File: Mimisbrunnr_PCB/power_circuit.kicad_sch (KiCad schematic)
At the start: 4 parts, among them J2 Jack-DC, U2 TLV76733DRVx

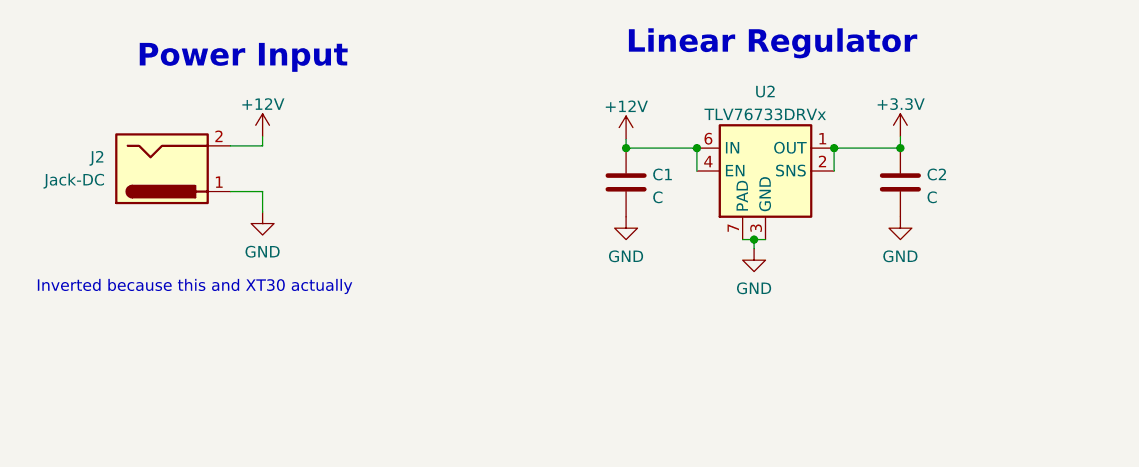
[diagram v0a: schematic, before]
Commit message: routing finished
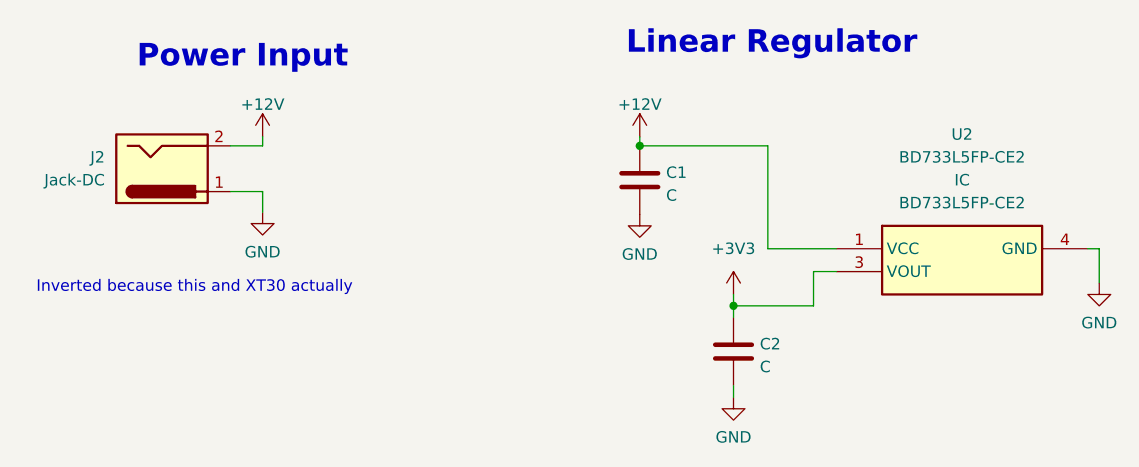
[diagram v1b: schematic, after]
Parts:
- removed U2: TLV76733DRVx, Package_TO_SOT_SMD:SOT-23-5_HandSoldering, symbol Regulator_Linear:TLV76733DRVx
- added U2: BD733L5FP-CE2, BD733L5FP:BD750L5FPCE2, symbol BD733L5FP:BD733L5FP-CE2
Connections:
- net +12V: now also U2.1 (VCC)
- net +3V3: now also U2.3 (VOUT)
- net GND: now also U2.4 (GND)
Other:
- moved on the sheet: C1
